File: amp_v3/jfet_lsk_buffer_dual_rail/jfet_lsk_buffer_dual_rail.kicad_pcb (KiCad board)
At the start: 2 copper layers, 83.8 x 30.5 mm, 29 parts, among them J3 AUDIO_IN, J4 PWR_IN, J8 AOUT_VACTROL, J9 AOUT_VIS, Q2 2N5457, Q4 2N5457

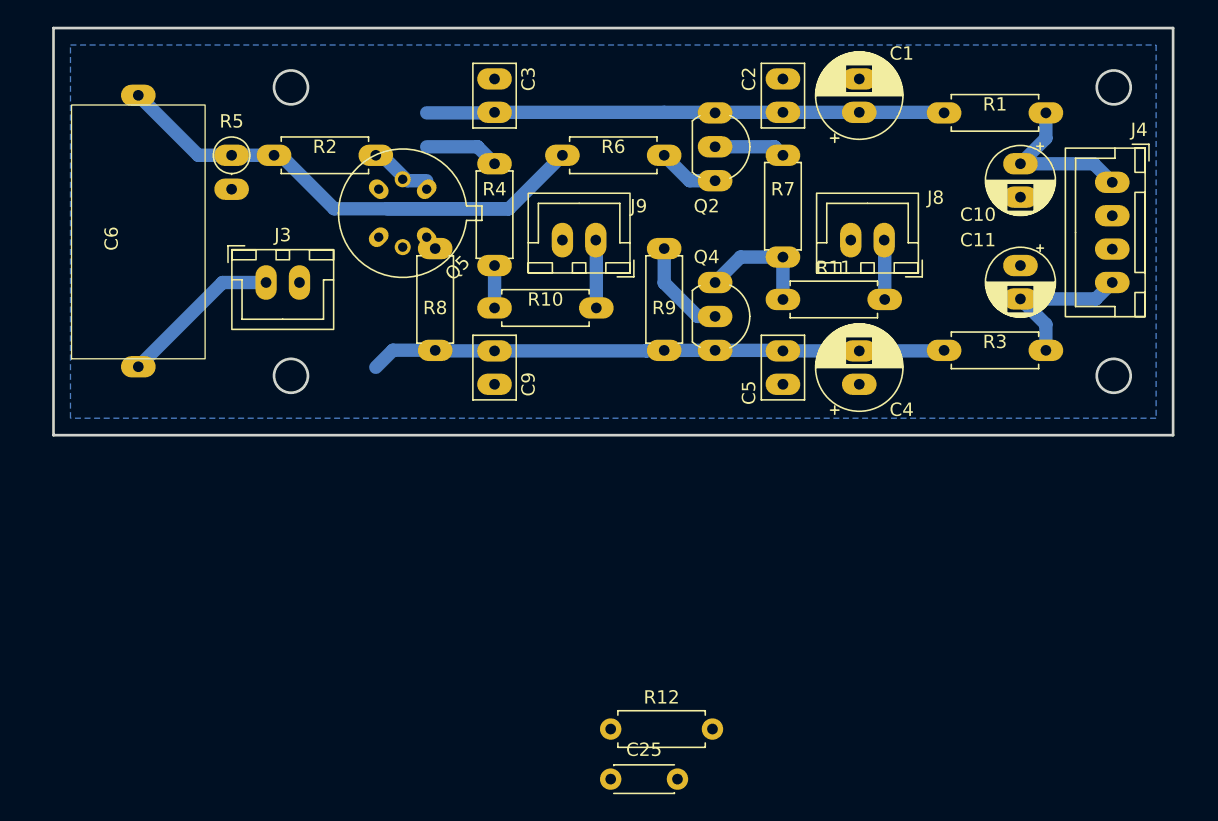
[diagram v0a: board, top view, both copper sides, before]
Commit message: updates
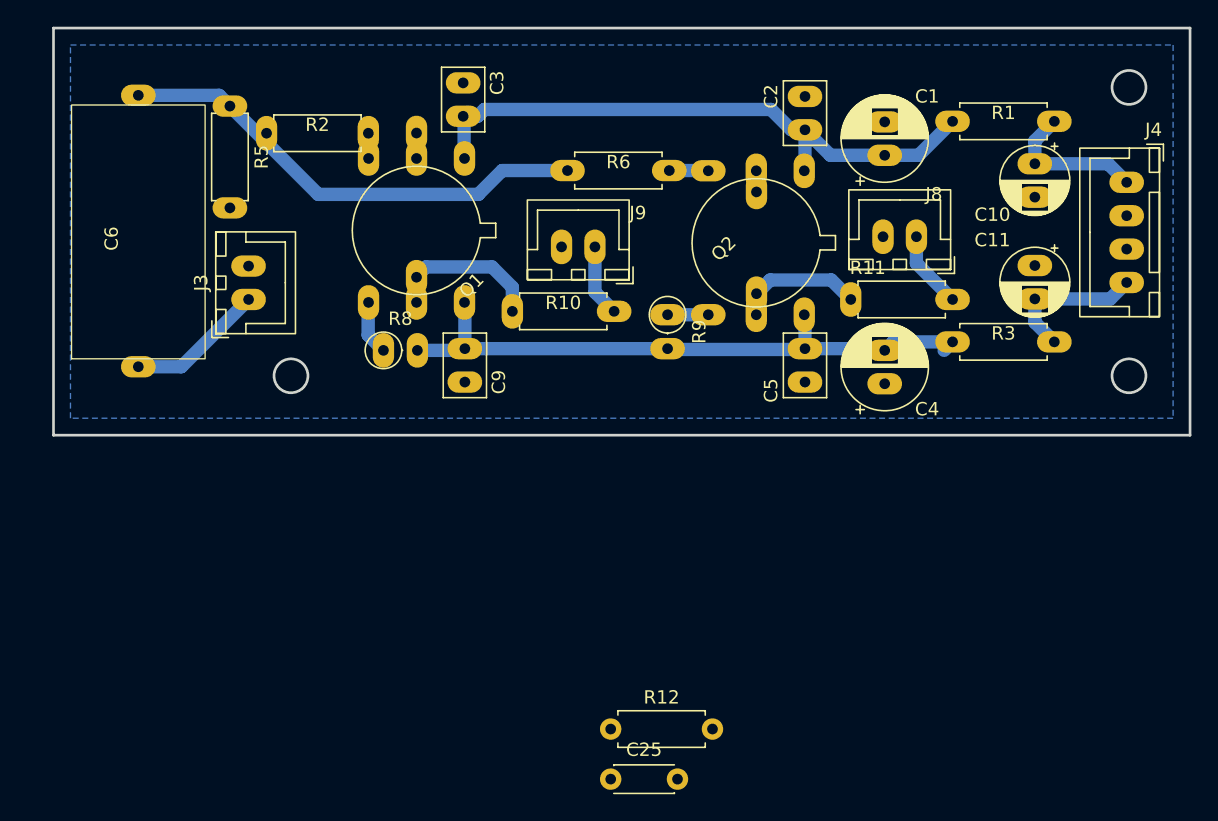
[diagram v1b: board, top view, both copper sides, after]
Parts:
- removed Q4: 2N5457, Package_TO_SOT_THT:TO-92L_Inline_Wide
- removed Q5: ~, Package_TO_SOT_THT:TO-75-6
- added Q1: ~, Package_TO_SOT_THT:TO-75-6, F.Cu at (132.5, 61.0)
- Q2: value 2N5457 -> ~; footprint Package_TO_SOT_THT:TO-92L_Inline_Wide -> Package_TO_SOT_THT:TO-75-6
- R4, R7: moved to B.Cu
- R5: footprint Resistor_THT:R_Axial_DIN0207_L6.3mm_D2.5mm_P2.54mm_Vertical -> Resistor_THT:R_Axial_DIN0207_L6.3mm_D2.5mm_P7.62mm_Horizontal
- R8, R9: footprint Resistor_THT:R_Axial_DIN0207_L6.3mm_D2.5mm_P7.62mm_Horizontal -> Resistor_THT:R_Axial_DIN0207_L6.3mm_D2.5mm_P2.54mm_Vertical
- moved Q2 9.31 mm to (157.9, 61.9), turned to -135 degrees
- moved R8 8.55 mm to (128.2, 71.8), turned to 0 degrees
- moved R4 5.86 mm to (130.7, 57.4)
- moved R11 5.08 mm to (163.2, 67.9)
- moved R9 4.96 mm to (149.5, 69.1)
- moved C1 3.74 mm to (165.7, 57.1)
- moved R5 3.69 mm to (116.7, 53.5)
- moved R7 3.38 mm to (156.1, 59.9)
- moved J8 2.43 mm to (168.1, 63.2)
- moved C3 2.37 mm to (134.2, 54.2)
- moved C9 2.23 mm to (134.3, 74.1)
- moved C2 2.11 mm to (159.8, 55.2)
- moved C4 1.91 mm to (165.7, 74.3)
- moved J3 1.82 mm to (118.1, 67.9), turned to 90 degrees
- moved R2 1.74 mm to (119.5, 55.5)
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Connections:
- R11 pad 1: Net-(Q4-D) -> Net-(Q2B-D)
- R7 pad 2: Net-(Q4-D) -> Net-(Q2B-D)
- R9 pad 1: Net-(Q4-S) -> Net-(Q2B-S)
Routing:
- net /AUDIO_IN: track 46.1 -> 36.0 mm
- net Net-(Q4-D): track 9.04 -> 0.00 mm
- net Net-(Q1B-D): track 3.17 -> 12.0 mm
- net Net-(Q2B-D): track 0.00 -> 8.09 mm
- net Net-(Q4-S): track 7.42 -> 0.00 mm
- net /+12VA: track 38.1 -> 45.3 mm
- net /-12VA: track 42.4 -> 48.0 mm
- net Net-(Q1A-D): track 5.61 -> 0.00 mm
- net Net-(Q2A-D): track 5.34 -> 0.00 mm
- net Net-(Q1A-G): track 4.60 -> 0.08 mm
- net Net-(Q1B-S): track 0.00 -> 3.98 mm
- net Net-(Q2B-S): track 0.00 -> 3.05 mm
- net /RCA_IN: track 12.2 -> 10.3 mm
- net Net-(Q2A-G): track 4.60 -> 2.93 mm
- net /OUT_B: track 4.40 -> 5.82 mm
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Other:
- board size 83.8 x 30.5 mm -> 85.1 x 30.5 mm

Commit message: inital
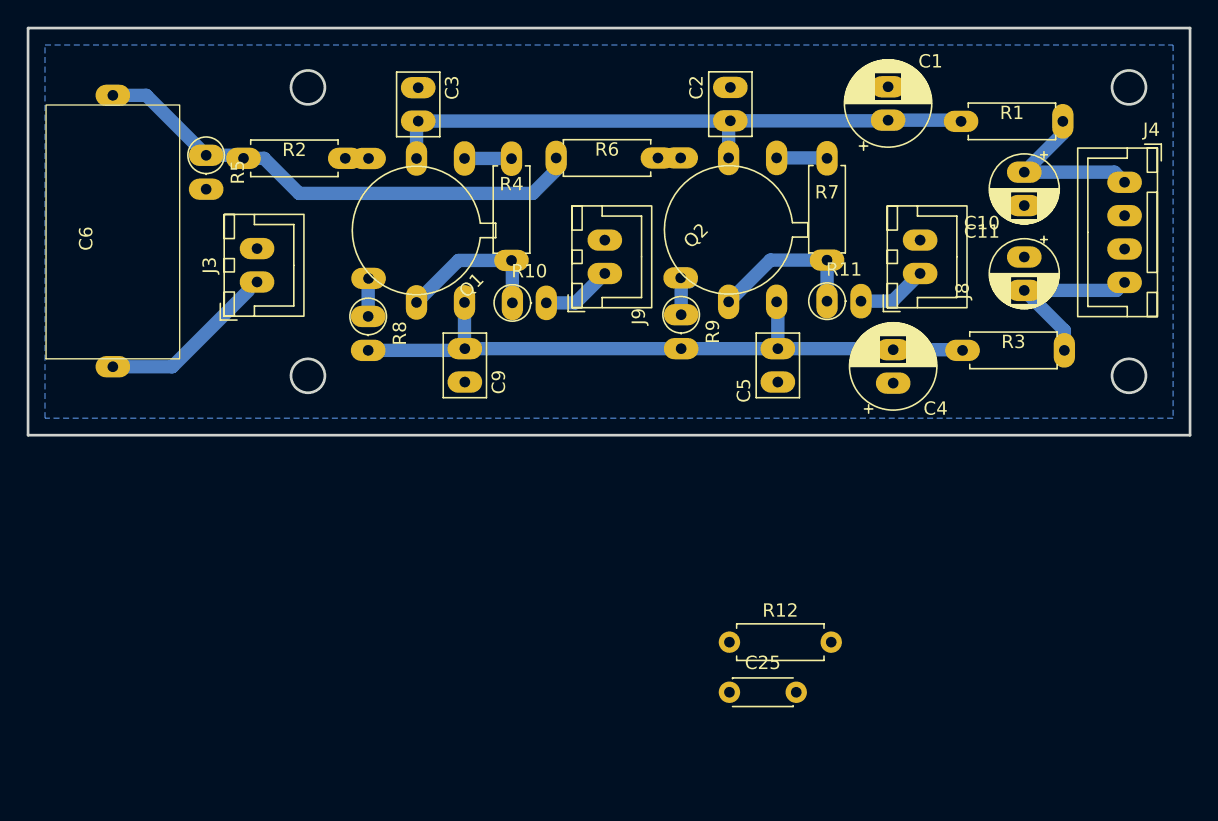
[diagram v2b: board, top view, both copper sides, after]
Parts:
- R10, R11, R5: footprint Resistor_THT:R_Axial_DIN0207_L6.3mm_D2.5mm_P7.62mm_Horizontal -> Resistor_THT:R_Axial_DIN0207_L6.3mm_D2.5mm_P2.54mm_Vertical
- R4, R7: value 68 -> 150; moved to F.Cu
- R8, R9: value 68 -> 150
- moved C25 11.0 mm to (154.1, 97.3)
- moved R12 11.0 mm to (154.1, 93.6)
- moved R4 7.11 mm to (137.8, 57.4)
- moved R7 5.85 mm to (161.4, 57.4)
- moved C2 5.63 mm to (154.2, 54.6)
- moved R5 4.09 mm to (114.9, 57.1)
- moved C3 3.38 mm to (130.8, 54.6)
- moved R8 2.79 mm to (127.1, 69.2), turned to -90 degrees
- moved J8 2.77 mm to (168.4, 66.0), turned to 90 degrees
- moved C1 2.64 mm to (166.0, 54.5)
- moved R2 2.55 mm to (117.7, 57.4)
- moved Q2 2.28 mm to (155.8, 60.9)
- moved J9 2.12 mm to (144.8, 66.0), turned to 90 degrees
- moved C5 2.03 mm to (157.7, 74.1)
- moved C6 1.91 mm to (108.0, 74.9)
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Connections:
- Q1 pad 1: /+12VA -> Net-(Q1A-S)
- Q1 pad 2: Net-(Q1A-D) -> /+12VA
- Q2 pad 1: /+12VA -> Net-(Q2A-S)
- Q2 pad 2: Net-(Q2A-D) -> /+12VA
- R4 pad 1: Net-(Q1A-D) -> Net-(Q1A-S)
- R7 pad 1: Net-(Q2A-D) -> Net-(Q2A-S)
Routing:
- net /-12VA: track 48.0 -> 52.1 mm
- net Net-(Q2A-S): track 0.00 -> 3.79 mm
- net Net-(Q2B-D): track 8.09 -> 11.7 mm
- net Net-(Q1A-S): track 0.00 -> 3.53 mm
- net Net-(Q2A-G): track 2.93 -> 0.15 mm
- net /-12V_IN: track 11.2 -> 13.5 mm
- net /RCA_IN: track 10.3 -> 12.5 mm
- net /AUDIO_IN: track 36.0 -> 38.0 mm
- net /+12V_IN: track 11.2 -> 12.8 mm
- net /+12VA: track 45.3 -> 46.6 mm
- net Net-(Q1B-S): track 3.98 -> 2.90 mm
- net /OUT_B: track 5.82 -> 5.29 mm
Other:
- board size 85.1 x 30.5 mm -> 87 x 30.5 mm
